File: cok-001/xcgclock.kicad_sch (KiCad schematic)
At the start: 24 parts, among them Y5001 14.31818MHz

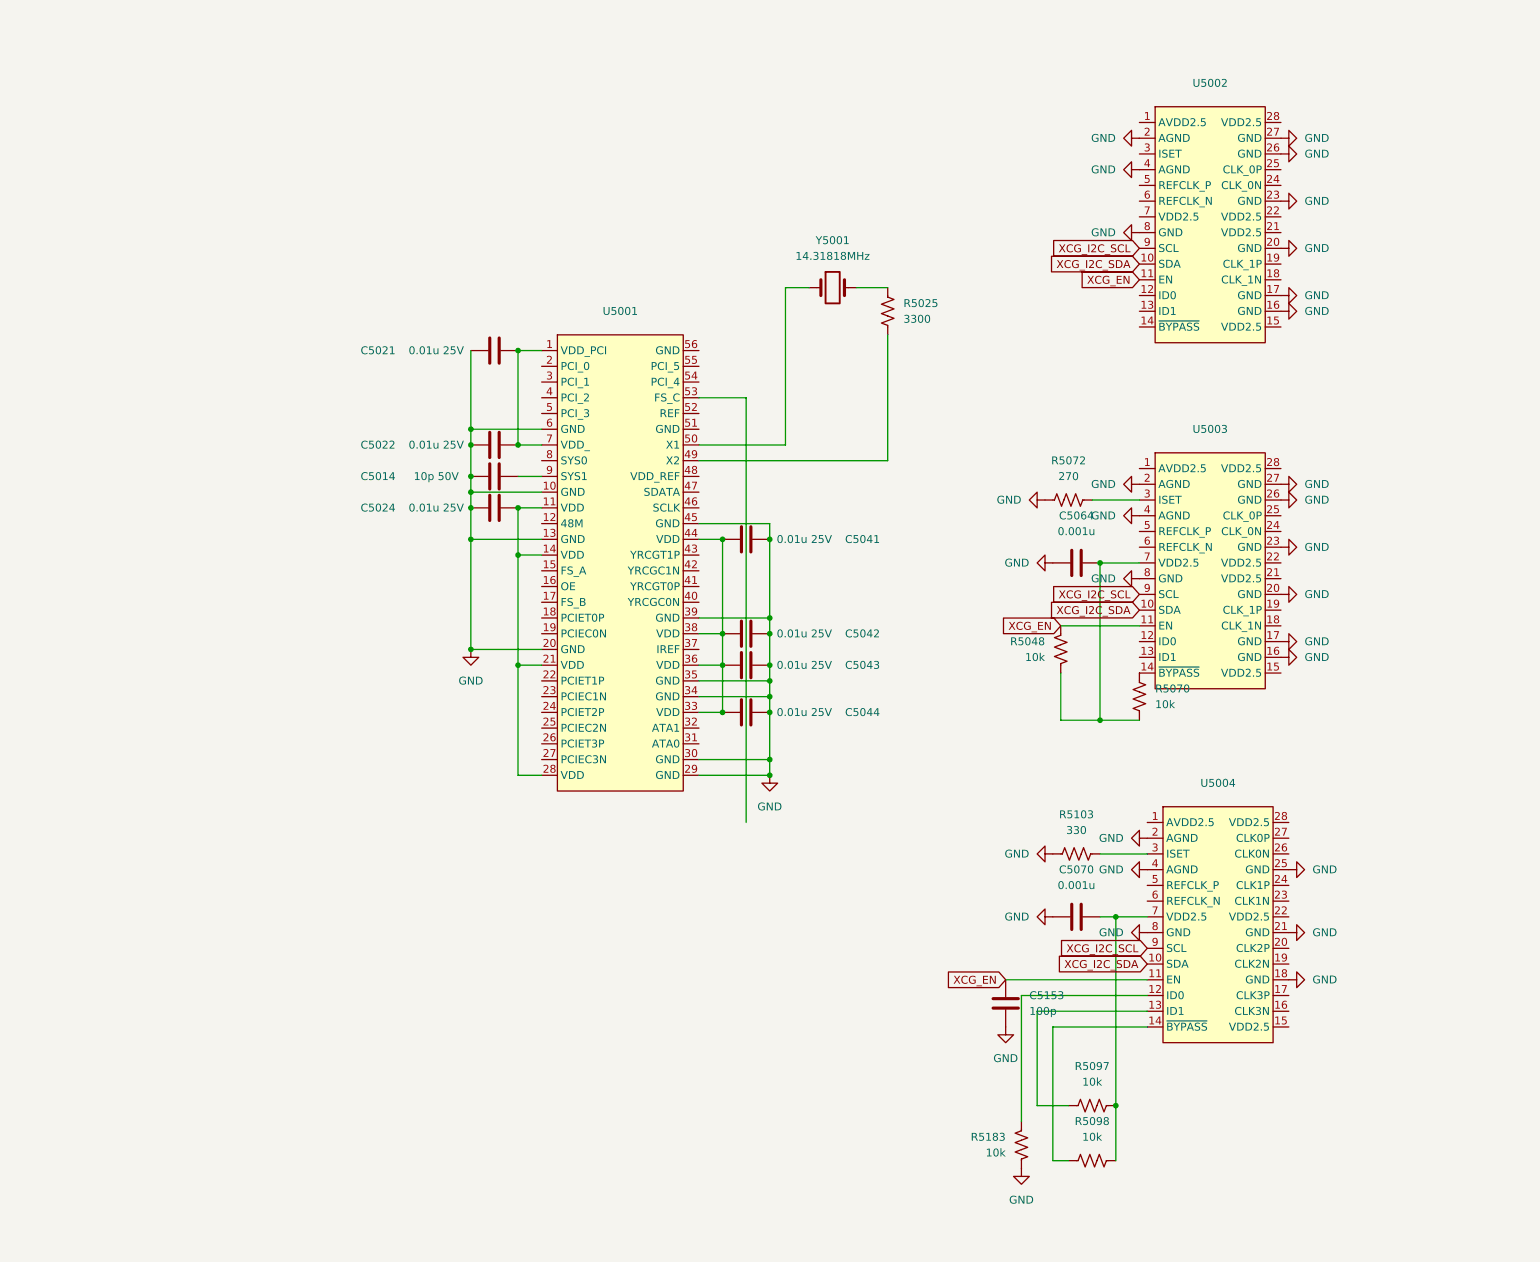
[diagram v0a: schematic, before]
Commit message: footprints
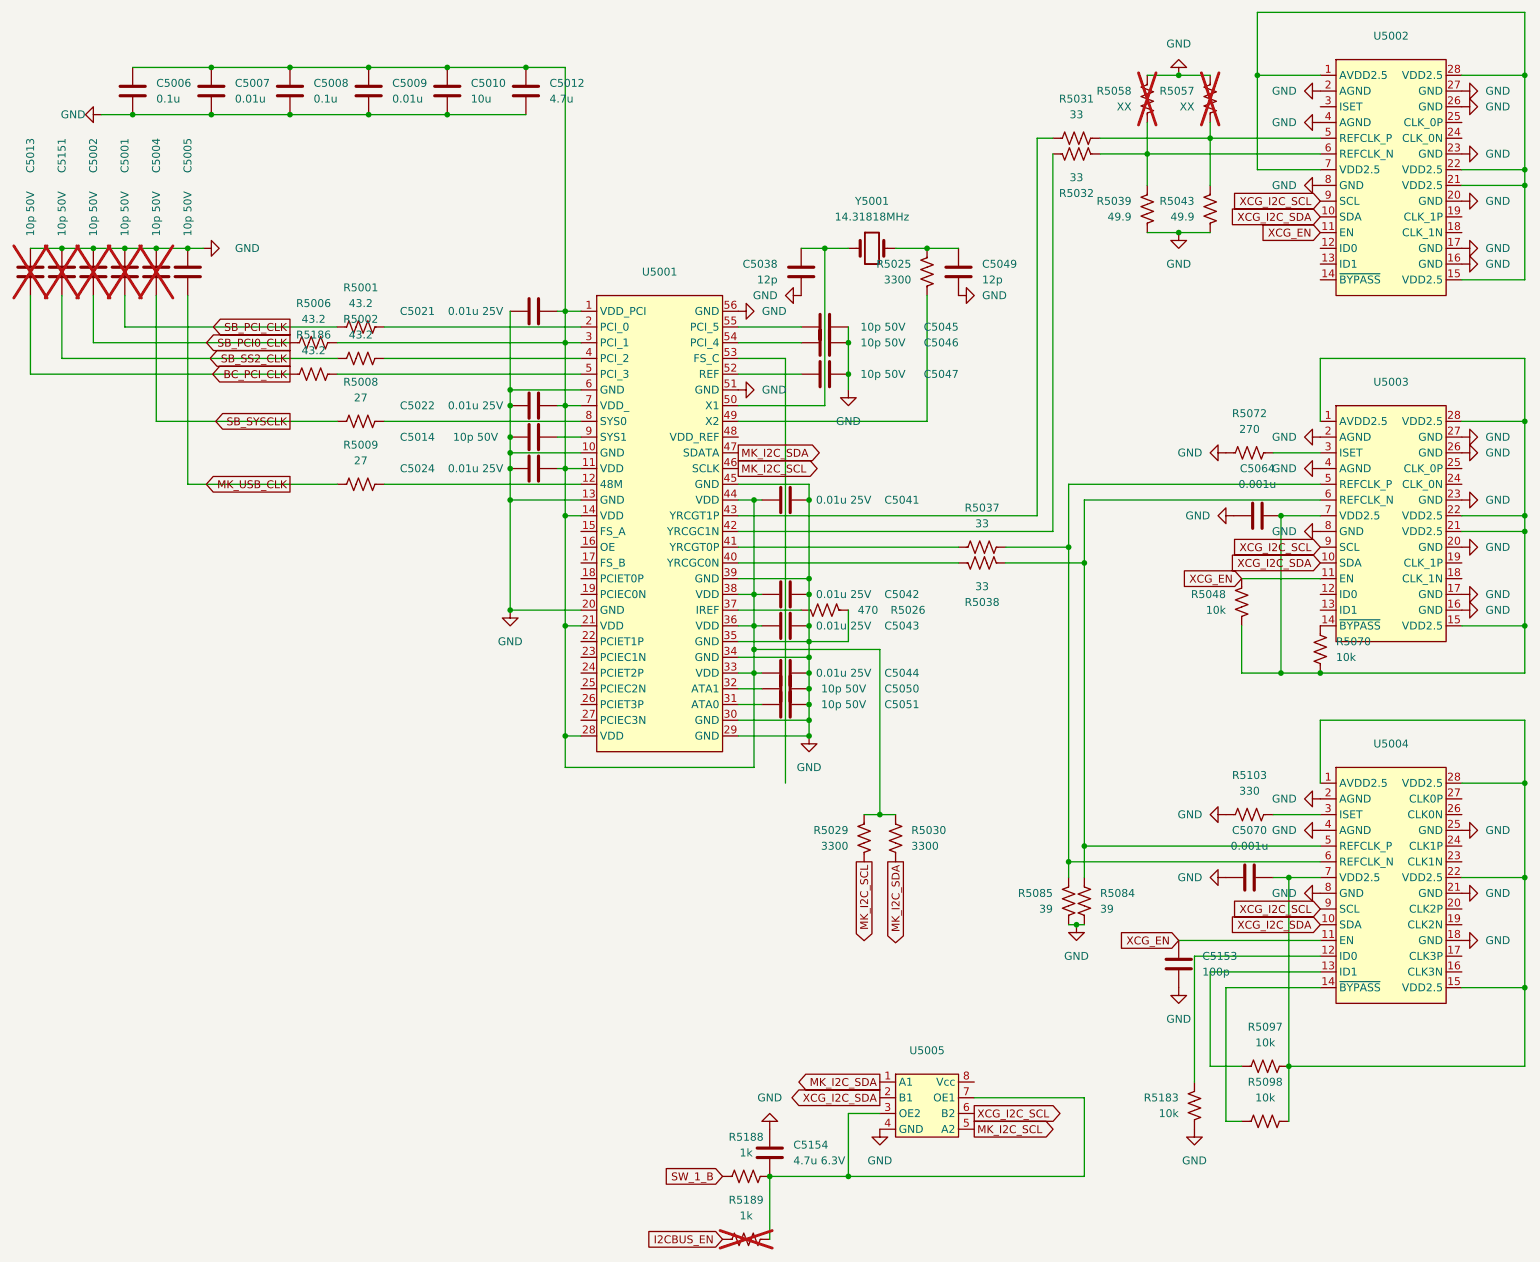
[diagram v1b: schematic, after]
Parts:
- added C5001, C5002, C5004, C5005, C5013, C5045, C5046, C5047, C5050, C5051, C5151: 10p 50V, Capacitor_SMD:C_0402_1005Metric, symbol Device:C
- added C5006, C5008: 0.1u, Capacitor_SMD:C_0402_1005Metric, symbol Device:C
- added C5007, C5009: 0.01u, Capacitor_SMD:C_0402_1005Metric, symbol Device:C
- added C5010: 10u, Capacitor_SMD:C_0402_1005Metric, symbol Device:C
- added C5012: 4.7u, Capacitor_SMD:C_0805_2012Metric, symbol Device:C
- added C5038, C5049: 12p, Capacitor_SMD:C_0402_1005Metric, symbol Device:C
- added C5154: 4.7u 6.3V, Capacitor_SMD:C_0603_1608Metric, symbol Device:C
- added R5001, R5002, R5006, R5186: 43.2, Resistor_SMD:R_0402_1005Metric, symbol Device:R_US
- added R5008, R5009: 27, Resistor_SMD:R_0402_1005Metric, symbol Device:R_US
- added R5026: 470, Resistor_SMD:R_0402_1005Metric, symbol Device:R_US
- added R5029, R5030: 3300, Resistor_SMD:R_0402_1005Metric, symbol Device:R_US
- added R5031, R5032, R5037, R5038: 33, Resistor_SMD:R_0402_1005Metric, symbol Device:R_US
- added R5039, R5043: 49.9, Resistor_SMD:R_0402_1005Metric, symbol Device:R_US
- added R5057, R5058: XX, Resistor_SMD:R_0402_1005Metric, symbol Device:R_US
- added R5084, R5085: 39, Resistor_SMD:R_0402_1005Metric, symbol Device:R_US
- added R5188, R5189: 1k, Resistor_SMD:R_0402_1005Metric, symbol Device:R_US
- added U5005: ~, Package_SO:VSSOP-8_2.3x2mm_P0.5mm, symbol PS3:TC7WB66FK
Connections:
- net GND: now also U5001.51 (GND), U5001.56 (GND), C5001.1, C5002.1, C5004.1, C5005.1, C5006.2, C5007.2, C5008.2, C5009.2, C5010.2, C5012.2, C5013.1, C5038.2, C5045.1, C5046.1, C5047.1, C5049.2, C5050.1, C5051.1, C5151.1, C5154.1, R5026.2, R5039.2, R5043.2, R5057.1, R5058.1, R5084.2, R5085.2, U5005.4 (GND)
- net XCG_I2C_SCL: now also U5005.6 (B2)
- net XCG_I2C_SDA: now also U5005.2 (B1)
- net at C5021.2, C5022.2, U5001.1 (VDD_PCI)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: now also C5024.2, C5041.2, C5042.2, C5043.2, C5044.2, U5001.11 (VDD), U5001.14 (VDD), U5001.21 (VDD), U5001.28 (VDD), U5001.3 (PCI_1), U5001.33 (VDD), U5001.36 (VDD), U5001.38 (VDD), U5001.44 (VDD), C5006.1, C5007.1, C5008.1, C5009.1, C5010.1, C5012.1, R5006.2, R5029.1, R5030.1
- net at R5025.1, Y5001.2: now also C5049.1
- net at C5070.2, R5097.2, R5098.2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: now also U5004.1 (AVDD2.5), U5004.15 (VDD2.5), U5004.22 (VDD2.5), U5004.28 (VDD2.5)
- net at U5001.50 (X1), Y5001.1: now also C5038.1
- net at U5002.1 (AVDD2.5): now also U5002.15 (VDD2.5), U5002.21 (VDD2.5), U5002.22 (VDD2.5), U5002.28 (VDD2.5), U5002.7 (VDD2.5)
- net at U5002.5 (REFCLK_P): now also R5031.2, R5043.1, R5057.2
- net at U5002.6 (REFCLK_N): now also R5032.2, R5039.1, R5058.2
- net at U5003.1 (AVDD2.5): now also C5064.2, R5048.1, R5070.1, U5003.15 (VDD2.5), U5003.21 (VDD2.5), U5003.22 (VDD2.5), U5003.28 (VDD2.5), U5003.7 (VDD2.5)
- net at U5003.5 (REFCLK_P): now also U5004.6 (REFCLK_N), R5037.2, R5085.1
- net at U5003.6 (REFCLK_N): now also U5004.5 (REFCLK_P), R5038.2, R5084.1
- net at U5001.12 (48M): now also R5009.2
- net at U5001.2 (PCI_0): now also R5001.2
- net at U5001.31 (ATA0): now also C5051.2
- net at U5001.32 (ATA1): now also C5050.2
- net at U5001.37 (IREF): now also R5026.1
- net at U5001.4 (PCI_2): now also R5002.2
- net at U5001.40 (YRCGC0N): now also R5038.1
- net at U5001.41 (YRCGT0P): now also R5037.1
- net at U5001.42 (YRCGC1N): now also R5032.1
- net at U5001.43 (YRCGT1P): now also R5031.1
- net MK_I2C_SCL: now reaches U5001.46 (SCLK)
- net MK_I2C_SCL: now also R5029.2, U5005.5 (A2)
- net MK_I2C_SDA: now reaches U5001.47 (SDATA)
- net MK_I2C_SDA: now also R5030.2, U5005.1 (A1)
- net at U5001.5 (PCI_3): now also R5186.2
- net at U5001.52 (REF): now also C5047.2
- net at U5001.54 (PCI_4): now also C5046.2
- net at U5001.55 (PCI_5): now also C5045.2
- net at U5001.8 (SYS0): now also R5008.2
- new net: C5154.2, R5188.2, R5189.2, U5005.3 (OE2), U5005.7 (OE1)
- new net BC_PCI_CLK: C5013.2, R5186.1
- new net I2CBUS_EN: R5189.1
- new net MK_USB_CLK: C5005.2, R5009.1
- new net SB_PCI0_CLK: C5002.2, R5006.1
- new net SB_PCI_CLK: C5001.2, R5001.1
- new net SB_SS2_CLK: C5151.2, R5002.1
- new net SB_SYSCLK: C5004.2, R5008.1
- new net SW_1_B: R5188.1
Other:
- moved on the sheet: C5014, C5021, C5022, C5024, C5041, C5042, C5043, C5044, C5064, C5070, C5153, R5025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
